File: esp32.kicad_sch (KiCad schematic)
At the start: 3 parts, among them U5 ESP32-WROOM-32

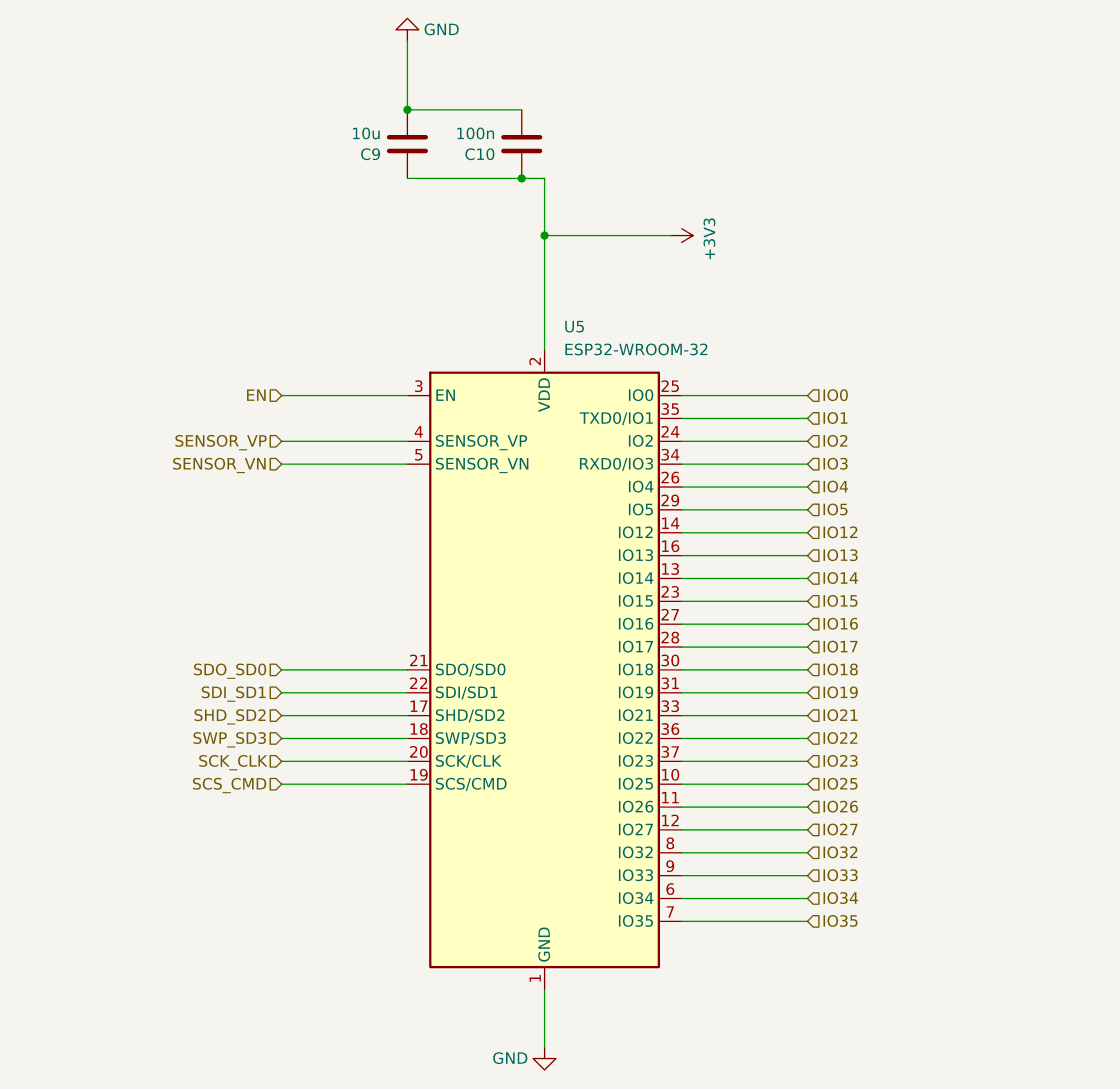
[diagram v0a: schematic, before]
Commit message: 1.01 WIP
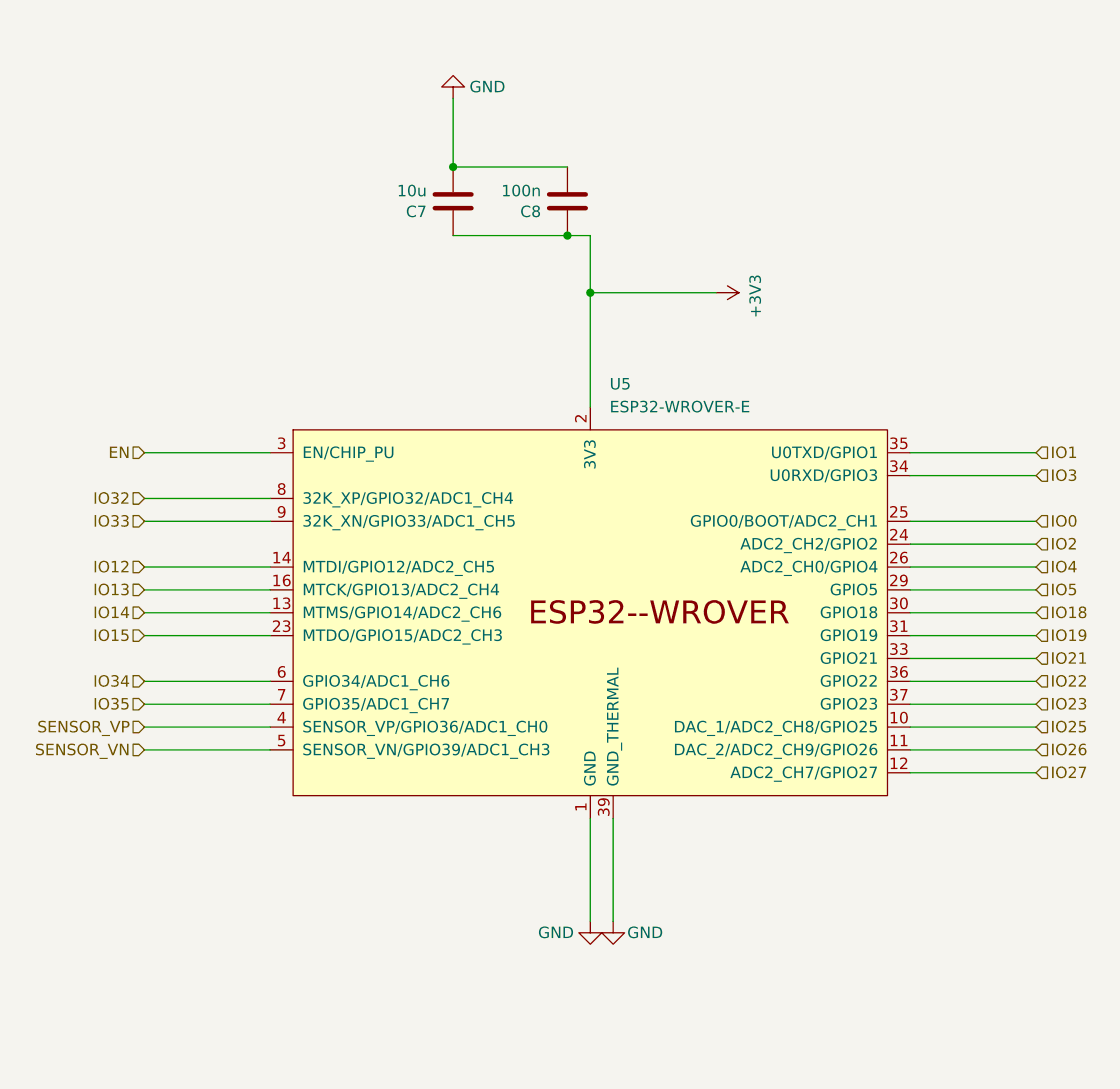
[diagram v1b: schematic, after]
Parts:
- removed C10: 100n, FRANK:Capacitor (0805), symbol Device:C
- removed C9: 10u, FRANK:Capacitor (0805), symbol Device:C
- removed U5: ESP32-WROOM-32, RF_Module:ESP32-WROOM-32, symbol RF_Module:ESP32-WROOM-32
- added C7: 10u, FRANK:Capacitor (0805), symbol Device:C
- added C8: 100n, FRANK:Capacitor (0805), symbol Device:C
- added U5: ESP32-WROVER-E, FRANK:ESP32-WROVER-E, symbol FRANK:ESP32-WROVER-E
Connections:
- net +3V3: now also C7.1, C8.1, U5.2 (3V3)
- net EN: now also U5.3 (EN/CHIP_PU)
- net GND: now also C7.2, C8.2, U5.1 (GND), U5.15 (GND), U5.38 (GND), U5.39 (GND_THERMAL)
- net IO0: now also U5.25 (GPIO0/BOOT/ADC2_CH1)
- net IO1: now also U5.35 (U0TXD/GPIO1)
- net IO12: now also U5.14 (MTDI/GPIO12/ADC2_CH5)
- net IO13: now also U5.16 (MTCK/GPIO13/ADC2_CH4)
- net IO14: now also U5.13 (MTMS/GPIO14/ADC2_CH6)
- net IO15: now also U5.23 (MTDO/GPIO15/ADC2_CH3)
- net IO18: now also U5.30 (GPIO18)
- net IO19: now also U5.31 (GPIO19)
- net IO2: now also U5.24 (ADC2_CH2/GPIO2)
- net IO21: now also U5.33 (GPIO21)
- net IO22: now also U5.36 (GPIO22)
- net IO23: now also U5.37 (GPIO23)
- net IO25: now also U5.10 (DAC_1/ADC2_CH8/GPIO25)
- net IO26: now also U5.11 (DAC_2/ADC2_CH9/GPIO26)
- net IO27: now also U5.12 (ADC2_CH7/GPIO27)
- net IO3: now also U5.34 (U0RXD/GPIO3)
- net IO32: now also U5.8 (32K_XP/GPIO32/ADC1_CH4)
- net IO33: now also U5.9 (32K_XN/GPIO33/ADC1_CH5)
- net IO34: now also U5.6 (GPIO34/ADC1_CH6)
- net IO35: now also U5.7 (GPIO35/ADC1_CH7)
- net IO4: now also U5.26 (ADC2_CH0/GPIO4)
- net IO5: now also U5.29 (GPIO5)
- net SENSOR_VN: now also U5.5 (SENSOR_VN/GPIO39/ADC1_CH3)
- net SENSOR_VP: now also U5.4 (SENSOR_VP/GPIO36/ADC1_CH0)
